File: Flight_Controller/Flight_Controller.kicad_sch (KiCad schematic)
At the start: 0 parts

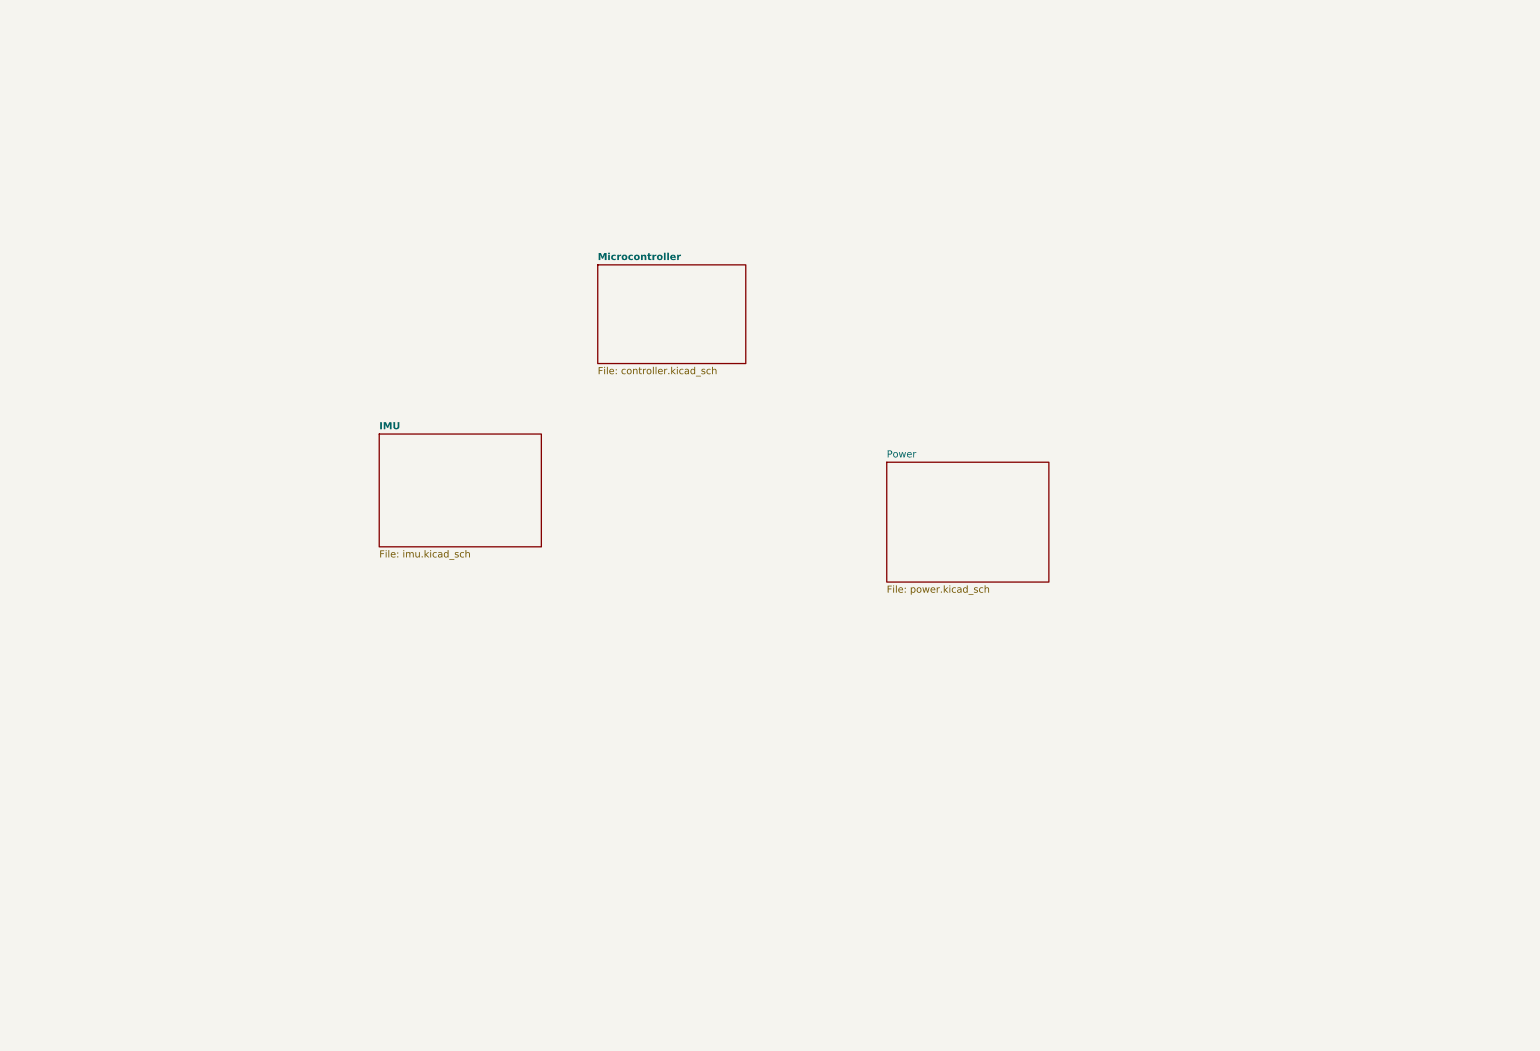
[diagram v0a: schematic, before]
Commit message: Rev 2 PCB done
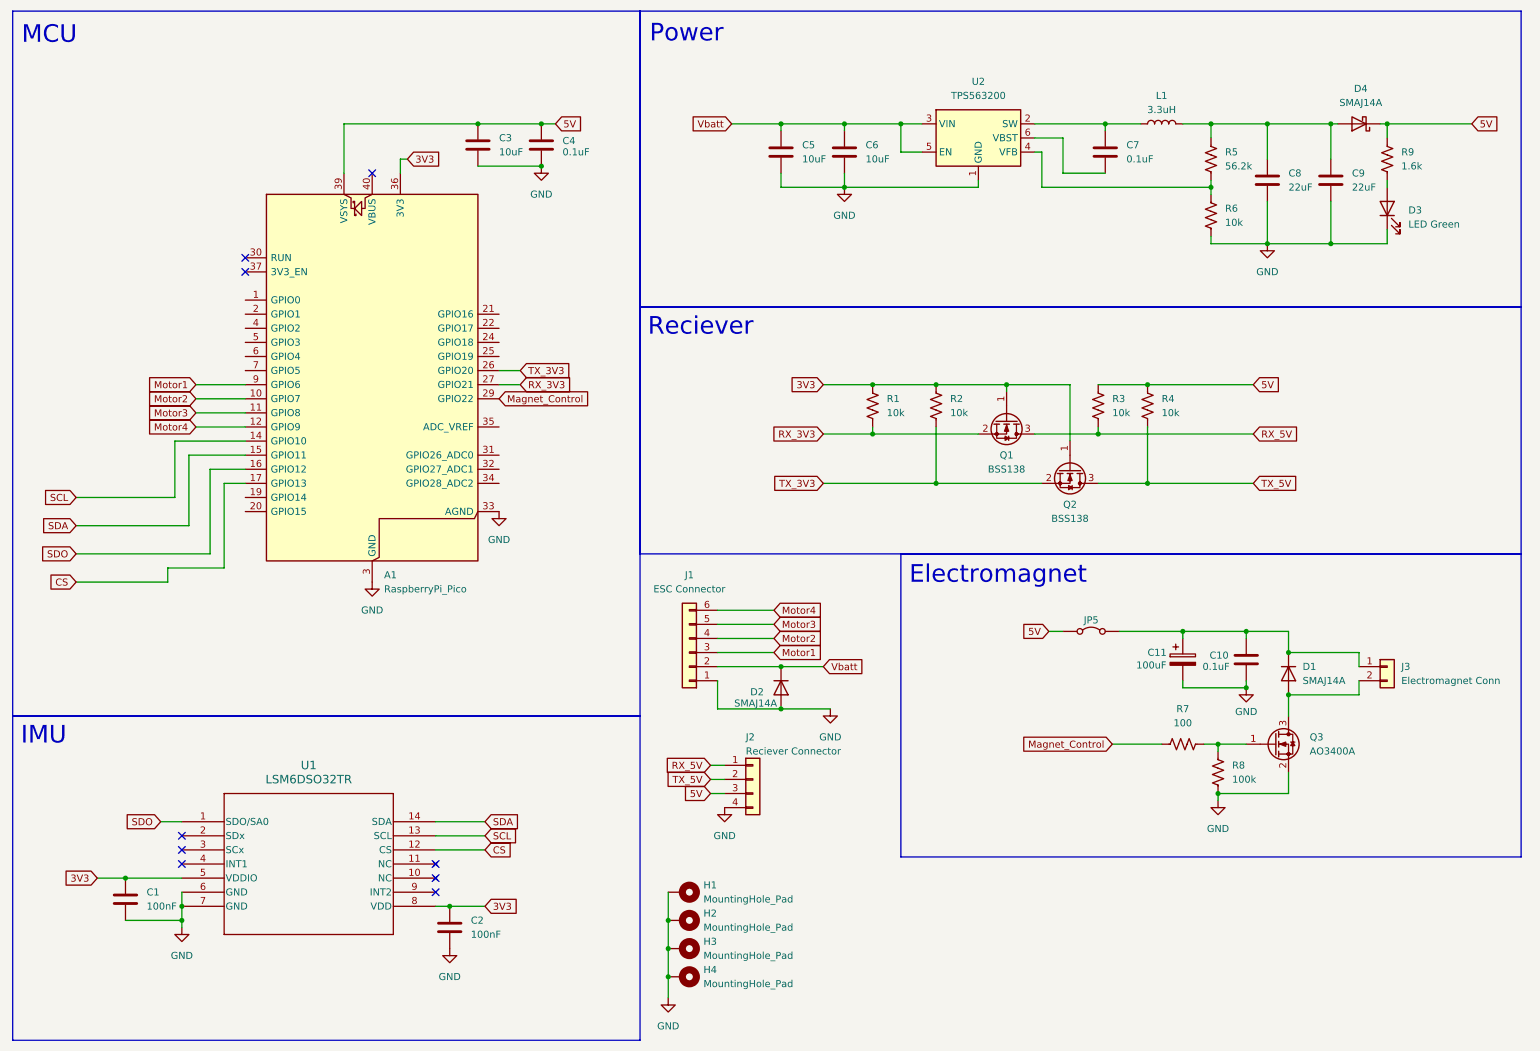
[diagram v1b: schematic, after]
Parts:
- added A1: RaspberryPi_Pico, Module:RaspberryPi_Pico_Common_SMD, symbol MCU_Module:RaspberryPi_Pico
- added C1, C2: 100nF, Capacitor_SMD:C_0603_1608Metric_Pad1.08x0.95mm_HandSolder, symbol Device:C
- added C10, C4, C7: 0.1uF, Capacitor_SMD:C_0603_1608Metric_Pad1.08x0.95mm_HandSolder, symbol Device:C
- added C11: 100uF, Capacitor_SMD:C_0603_1608Metric_Pad1.08x0.95mm_HandSolder, symbol Device:C_Polarized
- added C3, C5, C6: 10uF, Capacitor_SMD:C_0603_1608Metric_Pad1.08x0.95mm_HandSolder, symbol Device:C
- added C8, C9: 22uF, Capacitor_SMD:C_0603_1608Metric_Pad1.08x0.95mm_HandSolder, symbol Device:C
- added D1, D2: SMAJ14A, Diode_SMD:D_SMA_Handsoldering, symbol Device:D
- added D3: LED Green, Diode_SMD:D_0603_1608Metric_Pad1.05x0.95mm_HandSolder, symbol Device:LED
- added D4: SMAJ14A, Diode_SMD:D_SMA_Handsoldering, symbol Device:D_Schottky
- added H1, H2, H3, H4: MountingHole_Pad, MountingHole:MountingHole_3.5mm_Pad, symbol Mechanical:MountingHole_Pad
- added J1: ESC Connector, Connector_Wire:SolderWire-0.15sqmm_1x06_P4mm_D0.5mm_OD1.5mm_Relief, symbol Connector_Generic:Conn_01x06
- added J2: Reciever Connector, Alec_lib:Reciever_Module, symbol Connector_Generic:Conn_01x04
- added J3: Electromagnet Conn, Connector_Wire:SolderWire-0.15sqmm_1x02_P4mm_D0.5mm_OD1.5mm_Relief, symbol Connector_Generic:Conn_01x02
- added JP5: Jumper_2_Bridged, Jumper:SolderJumper-2_P1.3mm_Open_TrianglePad1.0x1.5mm, symbol Jumper:Jumper_2_Bridged
- added L1: 3.3uH, Inductor_SMD:L_Bourns-SRN8040_8x8.15mm, symbol Device:L
- added Q1, Q2: BSS138, Package_TO_SOT_SMD:SOT-23_Handsoldering, symbol Transistor_FET:BSS138
- added Q3: AO3400A, Package_TO_SOT_SMD:SOT-23, symbol Transistor_FET:AO3400A
- added R1, R2, R3, R4, R6: 10k, Resistor_SMD:R_0603_1608Metric_Pad0.98x0.95mm_HandSolder, symbol Device:R_US
- added R5: 56.2k, Resistor_SMD:R_0603_1608Metric_Pad0.98x0.95mm_HandSolder, symbol Device:R_US
- added R7: 100, Resistor_SMD:R_0603_1608Metric_Pad0.98x0.95mm_HandSolder, symbol Device:R_US
- added R8: 100k, Resistor_SMD:R_0603_1608Metric_Pad0.98x0.95mm_HandSolder, symbol Device:R_US
- added R9: 1.6k, Resistor_SMD:R_0603_1608Metric_Pad0.98x0.95mm_HandSolder, symbol Device:R_US
- added U1: LSM6DSO32TR, Package_LGA:LGA-14_3x2.5mm_P0.5mm_LayoutBorder3x4y, symbol Alecs_Lib:LSM6DSO32TR
- added U2: TPS563200, Package_TO_SOT_SMD:SOT-23-6, symbol Regulator_Switching:TPS563200
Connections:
- new net: C10.1, C11.1, D1.1 (K), J3.1 (Pin_1), JP5.2 (B)
- new net: D1.2 (A), J3.2 (Pin_2), Q3.3 (D)
- new net: Q3.1 (G), R7.2, R8.2
- new net: D3.2 (A), R9.2
- new net: C7.1, L1.1, U2.2 (SW)
- new net: C7.2, U2.6 (VBST)
- new net: C8.1, C9.1, D4.2 (A), L1.2, R5.1
- new net: R5.2, R6.1, U2.4 (VFB)
- new net 3V3: A1.36 (3V3), C1.1, C2.1, Q1.1 (G), Q2.1 (G), R1.1, R2.1, U1.5 (VDDIO), U1.8 (VDD)
- new net 5V: A1.39 (VSYS), C3.1, C4.1, D4.1 (K), J2.3 (Pin_3), JP5.1 (A), R3.1, R4.1, R9.1
- new net CS: A1.17 (GPIO13), U1.12 (CS)
- new net GND: A1.13 (GND), A1.18 (GND), A1.23 (GND), A1.28 (GND), A1.3 (GND), A1.33 (AGND), A1.38 (GND), A1.8 (GND), C1.2, C10.2, C11.2, C2.2, C3.2, C4.2, C5.2, C6.2, C8.2, C9.2, D2.2 (A), D3.1 (K), H1.1, H2.1, H3.1, H4.1, J1.1 (Pin_1), J2.4 (Pin_4), Q3.2 (S), R6.2, R8.1, U1.6 (GND), U1.7 (GND), U2.1 (GND)
- new net Magnet_Control: A1.29 (GPIO22), R7.1
- new net Motor1: A1.9 (GPIO6), J1.3 (Pin_3)
- new net Motor2: A1.10 (GPIO7), J1.4 (Pin_4)
- new net Motor3: A1.11 (GPIO8), J1.5 (Pin_5)
- new net Motor4: A1.12 (GPIO9), J1.6 (Pin_6)
- new net RX_3V3: A1.27 (GPIO21), Q1.2 (S), R1.2
- new net RX_5V: J2.1 (Pin_1), Q1.3 (D), R3.2
- new net SCL: A1.14 (GPIO10), U1.13 (SCL)
- new net SDA: A1.15 (GPIO11), U1.14 (SDA)
- new net SDO: A1.16 (GPIO12), U1.1 (SDO/SA0)
- new net TX_3V3: A1.26 (GPIO20), Q2.2 (S), R2.2
- new net TX_5V: J2.2 (Pin_2), Q2.3 (D), R4.2
- new net Vbatt: C5.1, C6.1, D2.1 (K), J1.2 (Pin_2), U2.3 (VIN), U2.5 (EN)
- no-connect marks 0 -> 9
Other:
- removed sheet IMU
- removed sheet Microcontroller
- removed sheet Power
- note added: "Electromagnet"
- note added: "IMU"
- note added: "MCU"
- note added: "Power"
- note added: "Reciever"
